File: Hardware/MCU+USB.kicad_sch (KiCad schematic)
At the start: 9 parts

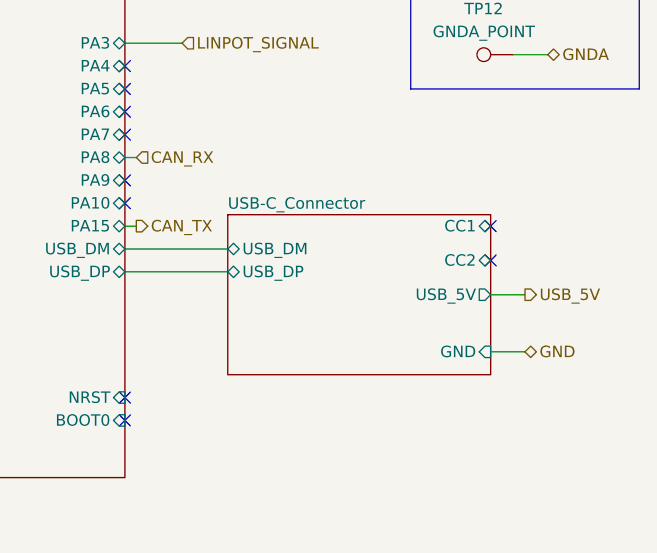
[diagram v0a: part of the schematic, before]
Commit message: Final Changes without Footprints
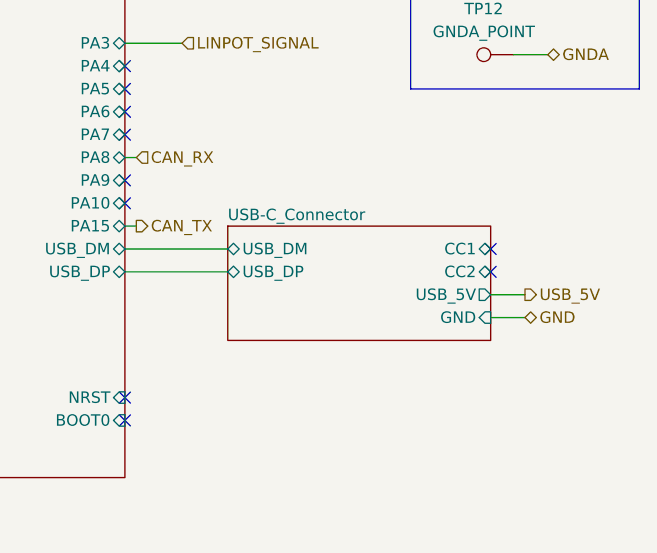
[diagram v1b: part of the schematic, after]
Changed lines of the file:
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@@
 	)
 	(no_connect
-		(at 144.78 80.01)
+		(at 144.78 81.28)
 	)
 	(no_connect
@@
 	)
 	(no_connect
-		(at 144.78 76.2)
+		(at 144.78 78.74)
 	)
 	(no_connect
@@
 	(wire
 		(pts
-			(xy 144.78 90.17) (xy 148.59 90.17)
+			(xy 144.78 86.36) (xy 148.59 86.36)
 		)
 		(stroke
@@
 	(hierarchical_label "GND"
 		(shape bidirectional)
-		(at 148.59 90.17 0)
+		(at 148.59 86.36 0)
 		(effects
 			(font
@@
 	)
 	(sheet
-		(at 115.57 74.93)
-		(size 29.21 17.78)
+		(at 115.57 76.2)
+		(size 29.21 12.7)
 		(exclude_from_sim no)
 		(in_bom yes)
@@
 		)
 		(property "Sheetname" "USB-C_Connector"
-			(at 115.57 74.422 0)
+			(at 115.57 75.692 0)
 			(show_name no)
 			(do_not_autoplace no)
@@
 		)
 		(property "Sheetfile" "USB-C_Connector.kicad_sch"
-			(at 115.57 93.218 0)
+			(at 115.57 94.488 0)
 			(hide yes)
 			(show_name no)
@@
 		)
 		(property "Author" "Shuopu Wang"
-			(at 87.63 -55.88 0)
+			(at 87.63 -54.61 0)
 			(hide yes)
 			(show_name no)
@@
 		)
 		(property "Date Modified" "9/5/2026"
-			(at 87.63 -55.88 0)
+			(at 87.63 -54.61 0)
 			(hide yes)
 			(show_name no)
@@
 		)
 		(pin "CC1" bidirectional
-			(at 144.78 76.2 0)
+			(at 144.78 78.74 0)
 			(effects
 				(font
@@
 		)
 		(pin "CC2" bidirectional
-			(at 144.78 80.01 0)
+			(at 144.78 81.28 0)
 			(effects
 				(font
@@
 		)
 		(pin "GND" input
-			(at 144.78 90.17 0)
+			(at 144.78 86.36 0)
 			(effects
 				(font
